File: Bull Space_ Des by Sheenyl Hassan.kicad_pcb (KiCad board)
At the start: 2 copper layers, 10 parts, among them IC1 TEENSY_4.0, IC2 XB24CZ7PIT-004, U1 Regulator_Linear_AP2204RB-3.3, U2 Flight-Computer_Adafruit_GPS_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, U3 ADXL343, U4 BMP280, U6 Memory_Flash_W25Q32JVSS

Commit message: Add files via upload
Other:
- net class Default removed

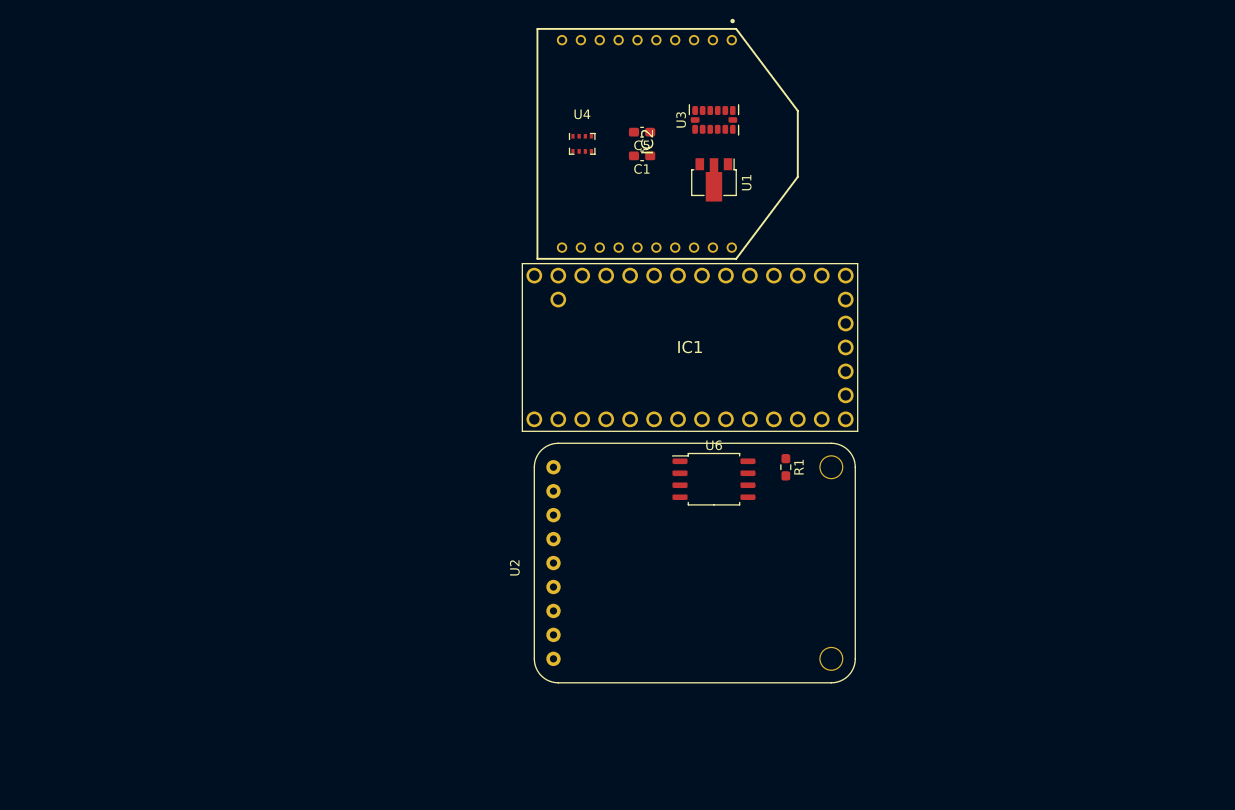
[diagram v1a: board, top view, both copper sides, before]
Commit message: Updates
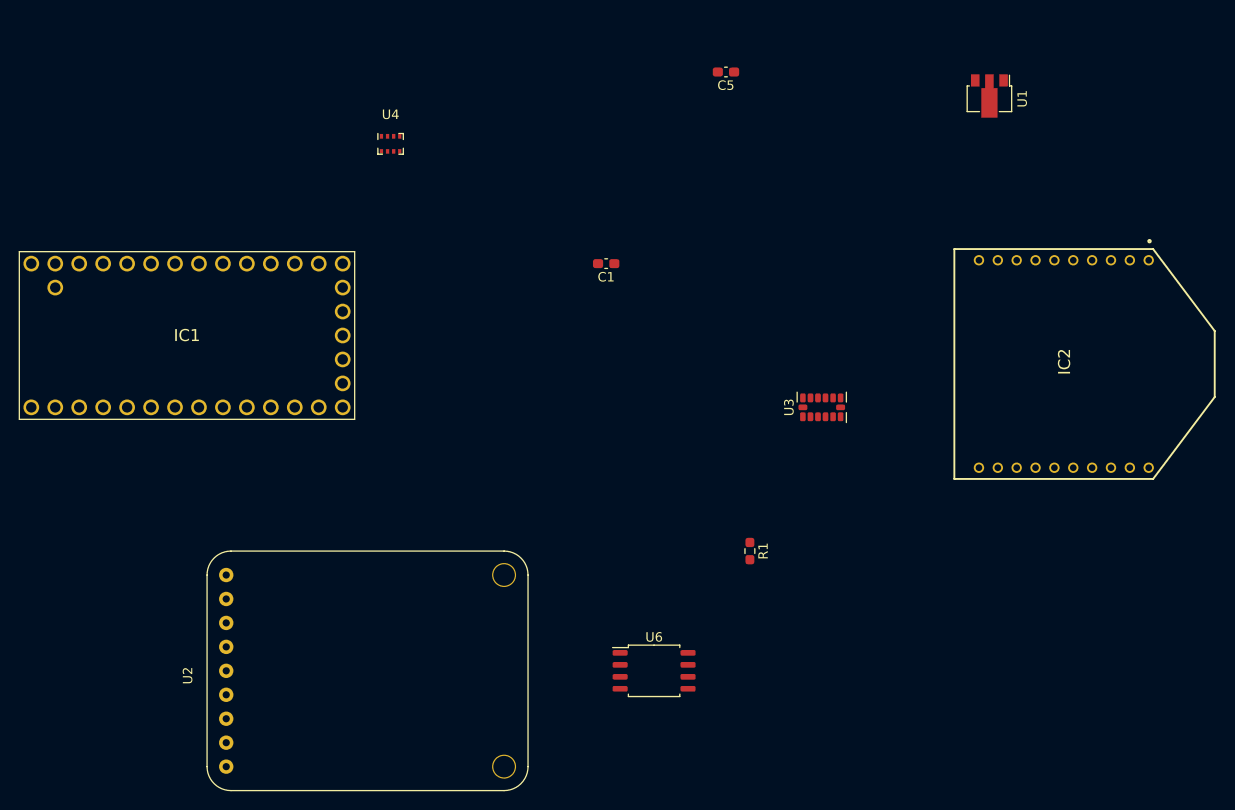
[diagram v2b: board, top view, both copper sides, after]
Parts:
- moved IC1 53.4 mm to (81.3, 114.3)
- moved IC2 50.0 mm to (206.8, 109.7)
- moved U2 36.5 mm to (99.9, 142.2)
- moved U3 32.6 mm to (165.1, 114.3)
- moved U1 30.5 mm to (182.9, 81.3)
- moved U6 21.3 mm to (147.3, 142.2)
- moved U4 20.3 mm to (119.4, 86.4)
- moved C1 12.0 mm to (142.2, 99.1)
- moved C5 10.9 mm to (154.9, 78.7)
- moved R1 9.67 mm to (157.5, 129.5)
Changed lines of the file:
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@@
   (net 68 "Net-(U2-Pad9)")
   (footprint "KiCad:TEENSY40" (layer "F.Cu")
-    (at 134.62 115.57)
+    (at 81.28 114.3)
     (descr "TEENSY 4.0-4")
     (tags "Integrated Circuit")
@@
   )
   (footprint "Package_LGA:LGA-14_3x5mm_P0.8mm_LayoutBorder1x6y" (layer "F.Cu")
-    (at 153.67 83.82 90)
+    (at 165.1 114.3 90)
     (descr "LGA, 14 Pin (http://www.st.com/resource/en/datasheet/lsm303dlhc.pdf), generated with kicad-footprint-generator ipc_noLead_generator.py")
     (tags "LGA NoLead")
@@
   )
   (footprint "Package_SO:SOIC-8_5.23x5.23mm_P1.27mm" (layer "F.Cu")
-    (at 153.67 121.92)
+    (at 147.32 142.24)
     (descr "SOIC, 8 Pin (http://www.winbond.com/resource-files/w25q32jv%20revg%2003272018%20plus.pdf#page=68), generated with kicad-footprint-generator ipc_gullwing_generator.py")
     (tags "SOIC SO")
@@
   )
   (footprint "Capacitor_SMD:C_0603_1608Metric_Pad1.08x0.95mm_HandSolder" (layer "F.Cu")
-    (at 146.05 87.63 180)
+    (at 142.24 99.06 180)
     (descr "Capacitor SMD 0603 (1608 Metric), square (rectangular) end terminal, IPC_7351 nominal with elongated pad for handsoldering. (Body size source: IPC-SM-782 page 76, https://www.pcb-3d.com/wordpress/wp-content/uploads/ipc-sm-782a_amendment_1_and_2.pdf), generated with kicad-footprint-generator")
     (tags "capacitor handsolder")
@@
   )
   (footprint "Capacitor_SMD:C_0603_1608Metric_Pad1.08x0.95mm_HandSolder" (layer "F.Cu")
-    (at 146.05 85.12 180)
+    (at 154.94 78.74 180)
     (descr "Capacitor SMD 0603 (1608 Metric), square (rectangular) end terminal, IPC_7351 nominal with elongated pad for handsoldering. (Body size source: IPC-SM-782 page 76, https://www.pcb-3d.com/wordpress/wp-content/uploads/ipc-sm-782a_amendment_1_and_2.pdf), generated with kicad-footprint-generator")
     (tags "capacitor handsolder")
@@
   )
   (footprint "Package_TO_SOT_SMD:SOT-89-3" (layer "F.Cu")
-    (at 153.67 90.17 -90)
+    (at 182.88 81.28 -90)
     (descr "SOT-89-3, http://ww1.microchip.com/downloads/en/DeviceDoc/3L_SOT-89_MB_C04-029C.pdf")
     (tags "SOT-89-3")
@@
   )
   (footprint "Resistor_SMD:R_0603_1608Metric_Pad0.98x0.95mm_HandSolder" (layer "F.Cu")
-    (at 161.29 120.65 -90)
+    (at 157.48 129.54 -90)
     (descr "Resistor SMD 0603 (1608 Metric), square (rectangular) end terminal, IPC_7351 nominal with elongated pad for handsoldering. (Body size source: IPC-SM-782 page 72, https://www.pcb-3d.com/wordpress/wp-content/uploads/ipc-sm-782a_amendment_1_and_2.pdf), generated with kicad-footprint-generator")
     (tags "resistor handsolder")
@@
   )
   (footprint "KiCad:XB24CAPIT-001" (layer "F.Cu")
-    (at 162.56 86.36 -90)
+    (at 206.77 109.702955 -90)
     (descr "Digi XBee 802.15.4")
     (tags "Integrated Circuit")
@@
   )
   (footprint "KiCad:Flight-Computer_Adafruit_GPS_THT_Footprint" (layer "F.Cu")
-    (at 134.62 130.81 -90)
+    (at 99.917 142.24 -90)
     (attr through_hole)
     (fp_text reference "U2" (at 0.508 2.032 90) (layer "F.SilkS")
@@
   )
   (footprint "Package_LGA:Bosch_LGA-8_2x2.5mm_P0.65mm_ClockwisePinNumbering" (layer "F.Cu")
-    (at 139.7 86.36)
+    (at 119.38 86.36)
     (descr "LGA-8, https://ae-bst.resource.bosch.com/media/_tech/media/datasheets/BST-BMP280-DS001-18.pdf")
     (tags "lga land grid array")
